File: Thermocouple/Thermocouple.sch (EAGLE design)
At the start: 20 parts, among them Q2 BSS138

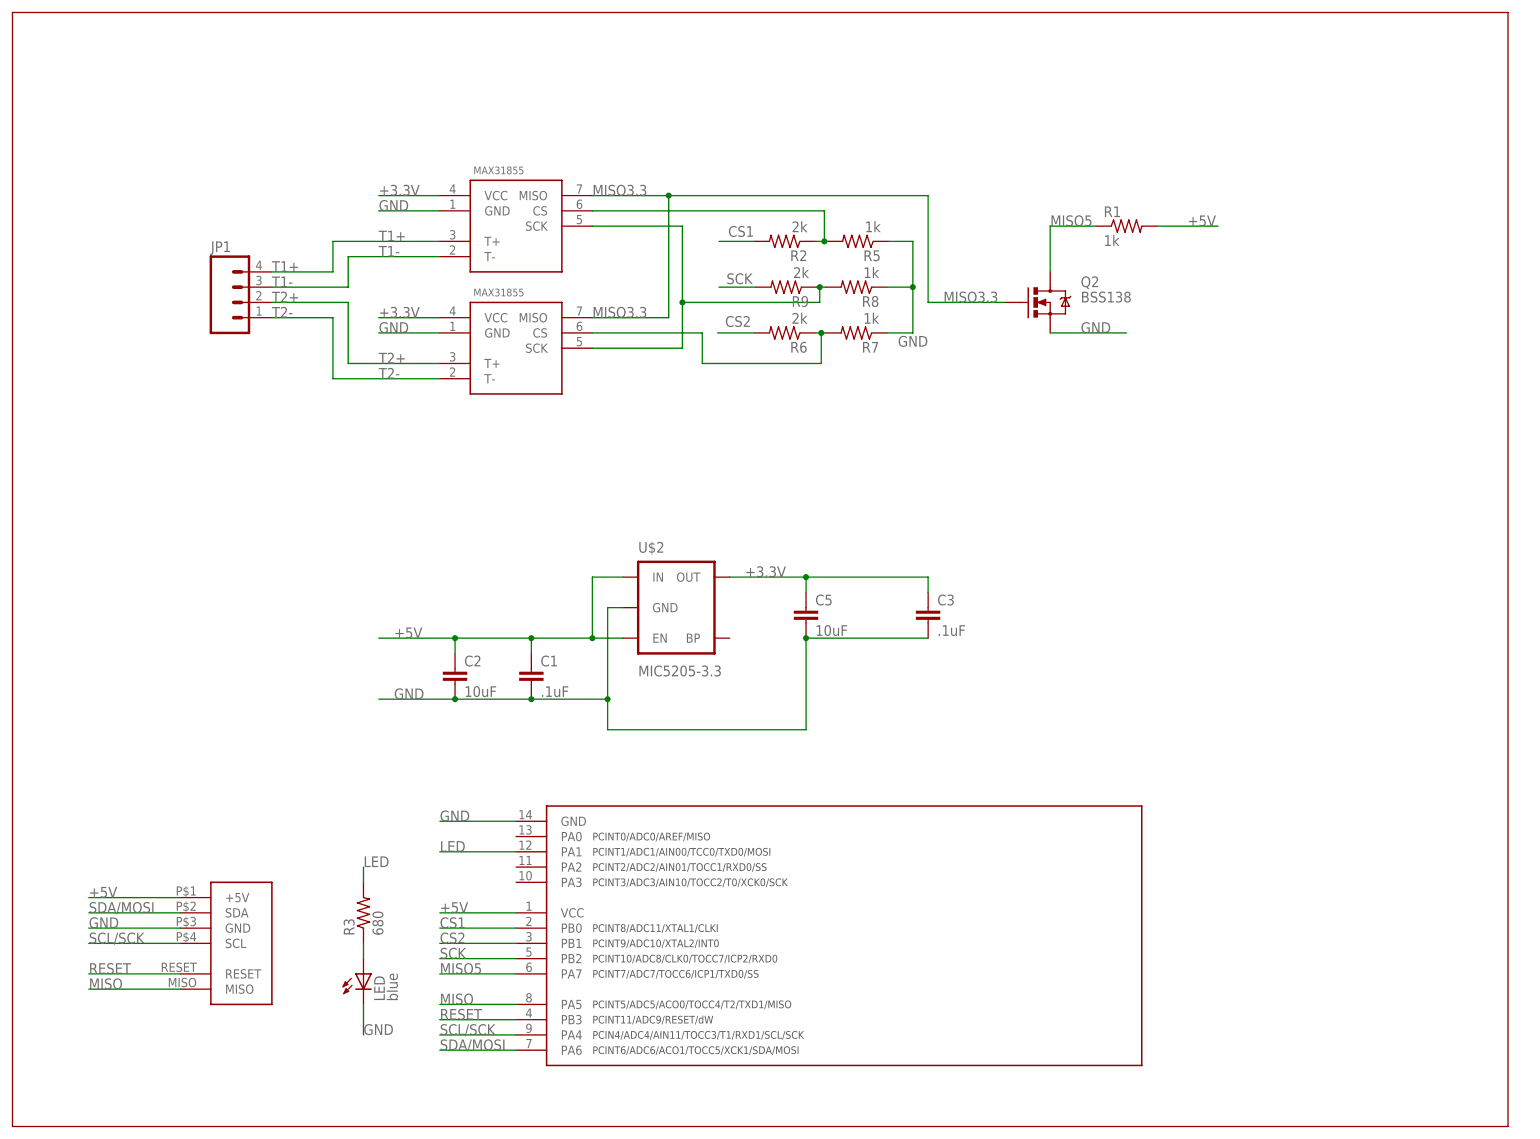
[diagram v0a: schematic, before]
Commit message: Latest version of schematics and boards
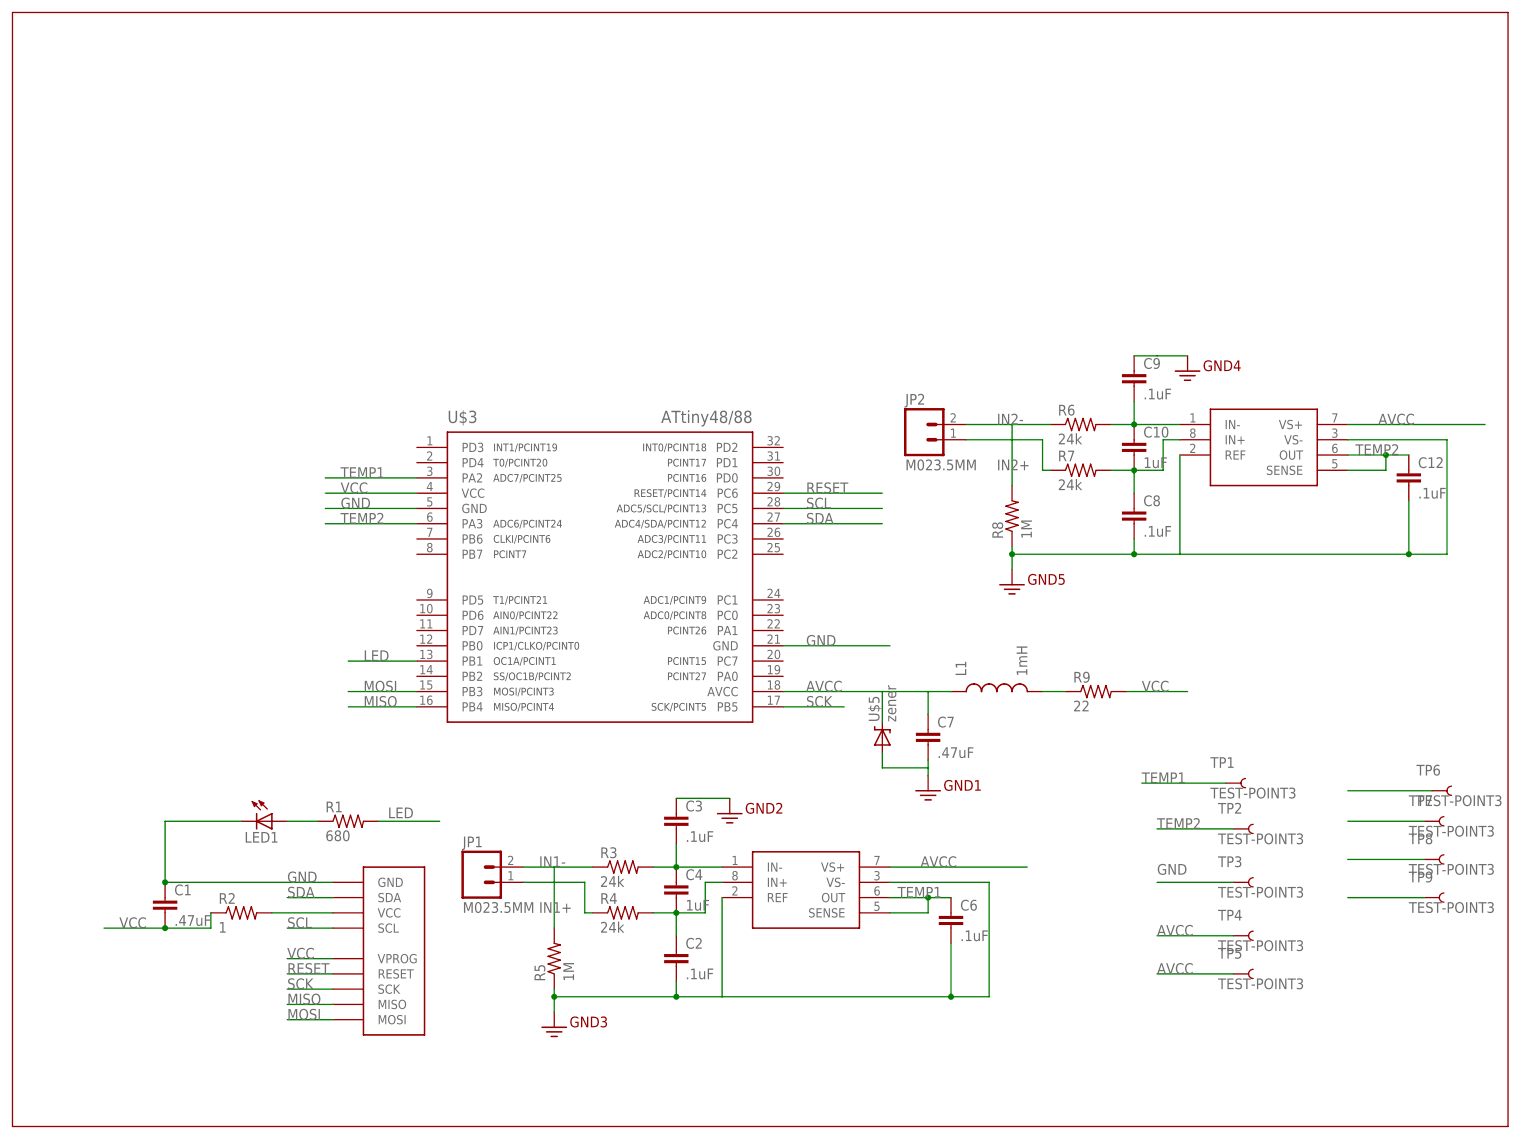
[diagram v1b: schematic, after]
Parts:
- removed C5: 10uF, SparkFun-Capacitors:CAP0805
- removed LED: blue, led:LEDCHIPLED_1206
- removed Q2: BSS138, SparkFun-DiscreteSemi:MOSFET-NCHANNELBSS138
- added C10, C4: 1uF, SparkFun-Capacitors:CAP0805
- added C12, C6, C8, C9: .1uF, SparkFun-Capacitors:CAP0805
- added C7: .47uF, SparkFun-Capacitors:CAP0805
- added JP2: M023.5MM, SparkFun-Connectors:M023.5MM
- added L1: 1mH, SparkFun-Passives:INDUCTOR1007
- added LED1: (no value), adafruit:LEDCHIP-LED0805
- added R4: 24k, SparkFun-Resistors:RESISTOR0805-RES
- added TP1, TP2, TP3, TP4, TP5, TP6, TP7, TP8, TP9: TEST-POINT3, SparkFun-Passives:TEST-POINT3
- C1: value .1uF -> .47uF
- C2: value 10uF -> .1uF
- JP1: value (none) -> M023.5MM; device SparkFun-Connectors:M04SCREW -> SparkFun-Connectors:M023.5MM
- R1: value 1k -> 680; device SparkFun-Resistors:RESISTOR0805-RES -> SparkFun-Passives:RESISTOR0805-RES
- R2: value 2k -> 1
- R3: value 680 -> 24k; device SparkFun-Passives:RESISTOR0805-RES -> SparkFun-Resistors:RESISTOR0805-RES
- R5, R8: value 1k -> 1M
- R6: value 2k -> 24k
- R7: value 1k -> 24k
- R9: value 2k -> 22; device SparkFun-Resistors:RESISTOR0805-RES -> SparkFun-Passives:RESISTOR0805-RES
- U$1: value MAX31855 -> AD8495; device IntegerLabs:MAX31855 -> IntegerLabs:AD8495
- U$2: value MIC5205-3.3 -> FOOTPRINTFOOTPRINT-2; device SparkFun-PowerIC:V_REG_MIC52053.3V -> IntegerLabs:FOOTPRINTFOOTPRINT-2
- U$3: value TINY841 -> ATTINY48/88-TQFP; device IntegerLabs:TINY841 -> IntegerLabs:ATTINY48/88-TQFP
- U$4: value FOOTPRINT -> AD8495; device IntegerLabs:FOOTPRINT -> IntegerLabs:AD8495
- U$5: value MAX31855 -> zener; device IntegerLabs:MAX31855 -> SparkFun-DiscreteSemi:DIODE-ZENER-BZT52
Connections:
- removed net +3.3V: C3.1, C5.1, U$1.VCC, U$2.OUT, U$5.VCC
- removed net +5V: C1.1, C2.1, R1.2, U$2.EN, U$2.IN, U$3.VCC, U$4.+5V
- removed net CS1: R2.2, U$3.PB0
- removed net CS1-3.3: R2.1, R5.2, U$1.CS
- removed net CS2: R6.2, U$3.PB1
- removed net CS2-3.3: R6.1, R7.2, U$5.CS
- removed net MISO3.3: Q2.G, U$1.MISO, U$5.MISO
- removed net MISO5: Q2.D, R1.1, U$3.PA7
- removed net SCK-3.3: R8.2, R9.1, U$1.SCK, U$5.SCK
- removed net SCL/SCK: U$3.PA4, U$4.SCL
- removed net SDA/MOSI: U$3.PA6, U$4.SDA
- removed net T1+: JP1.4, U$1.T+
- removed net T1-: JP1.3, U$1.T-
- removed net T2+: JP1.2, U$5.T+
- removed net T2-: JP1.1, U$5.T-
- new net AVCC: C7.1, L1.1, TP4.1, TP5.1, U$1.VS+, U$3.AVCC, U$4.VS+, U$5.C
- new net IN1+: JP1.1, R4.1, TP6.1
- new net IN1-: JP1.2, R3.1, R5.2, TP7.1
- new net IN2+: JP2.1, R7.1, TP8.1
- new net IN2-: JP2.2, R6.1, R8.2, TP9.1
- new net MOSI: U$2.MOSI, U$3.PB3
- new net N$2: R2.2, U$2.VCC
- new net N$3: C3.2, C4.1, R3.2, U$1.IN-
- new net N$4: C2.1, C4.2, R4.2, U$1.IN+
- new net N$6: C10.2, C8.1, R7.2, U$4.IN+
- new net N$7: L1.2, R9.1
- new net N$8: LED1.A, R1.1
- new net SCL: U$2.SCL, U$3.PC5
- new net SDA: U$2.SDA, U$3.PC4
- new net TEMP1: C6.1, TP1.1, U$1.OUT, U$1.SENSE, U$3.PA2
- new net TEMP2: C12.1, TP2.1, U$3.PA3, U$4.OUT, U$4.SENSE
- new net VCC: C1.2, R2.1, R9.2, U$2.VPROG, U$3.VCC
- net GND: now also C1.1, C12.2, C3.1, C6.2, C7.2, C8.2, C9.1, LED1.C, TP3.1, U$1.REF, U$1.VS-, U$3.GND@1, U$4.REF, U$4.VS-, U$5.A; no longer C1.2, C3.2, C5.2, LED.C, Q2.S, R7.1, U$1.GND, U$4.GND, U$5.GND
- net LED: now also R1.2, U$3.PB1; no longer R3.2, U$3.PA1
- net MISO: now also U$2.MISO, U$3.PB4; no longer U$3.PA5, U$4.MISO
- net N$5: now also C10.1, C9.2, R6.2, U$4.IN-; no longer LED.A, R3.1
- net RESET: now also U$2.RESET, U$3.PC6; no longer U$3.PB3, U$4.RESET
- net SCK: now also U$2.SCK, U$3.PB5; no longer R9.2, U$3.PB2
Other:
- moved on the sheet: C1, C2, C3, R1, R2, R3, R5, R6, R7, R8, R9
